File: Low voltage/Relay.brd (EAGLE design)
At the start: 100 x 80 mm, 9 parts, among them T1 2N1613

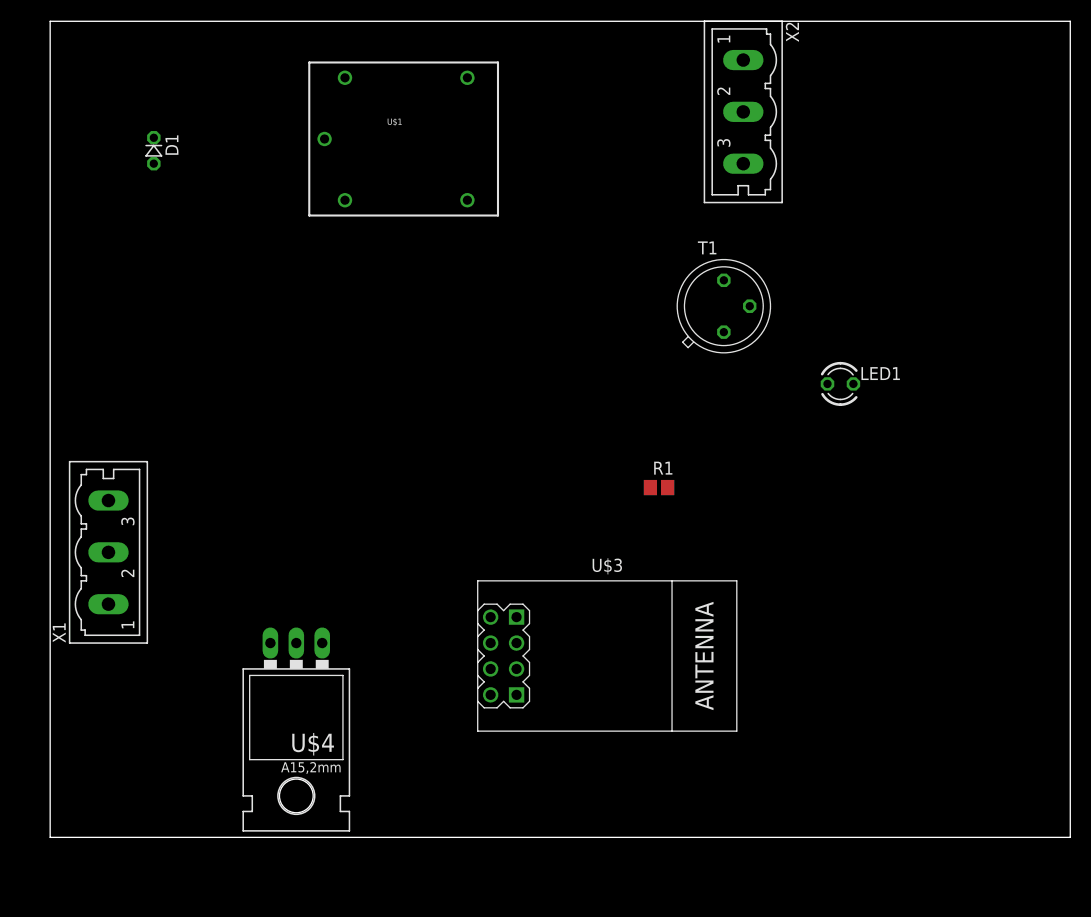
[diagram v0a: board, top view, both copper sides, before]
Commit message: board layout
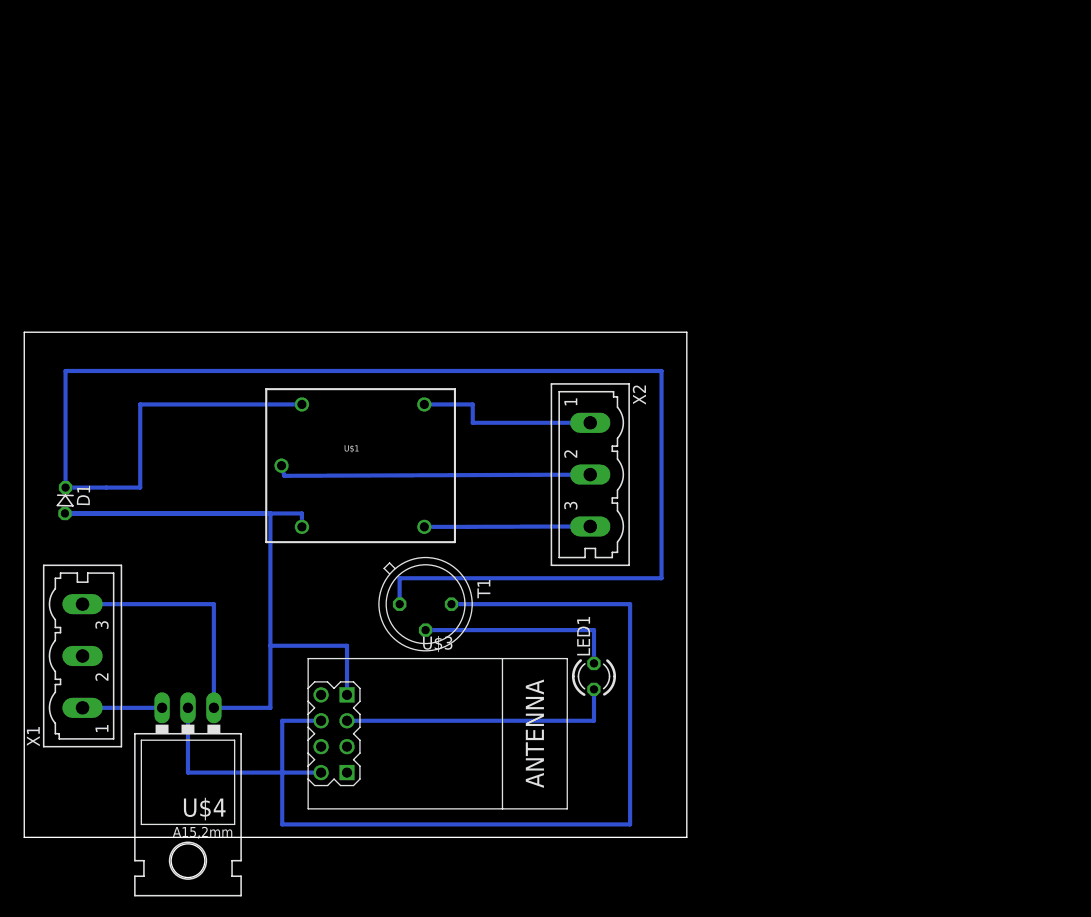
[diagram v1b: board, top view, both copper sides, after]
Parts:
- removed R1: 1k, resistor:R2012
- moved T1 41.3 mm to (36.8, 22.9), turned to 270 degrees
- moved X2 38.6 mm to (53.6, 35.6)
- moved LED1 37.5 mm to (53.3, 15.8), turned to 90 degrees
- moved D1 35.4 mm to (1.48, 33.0), turned to 268.7 degrees
- moved U$1 32.3 mm to (30.1, 36.6)
- moved U$3 18.3 mm to (38.0, 10.2)
- moved U$4 12.4 mm to (13.5, 8.89)
- moved X1 10.5 mm to (2.54, 17.8)
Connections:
- removed net N$3: LED1.A, R1.2
- net N$2: now also LED1.A; no longer R1.1
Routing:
- net N$8: track 0.00 -> 149.7 mm
- net N$1: track 0.00 -> 106.6 mm
- net GND: track 0.00 -> 104.6 mm
- net N$9: track 0.00 -> 31.0 mm
- net N$2: track 0.00 -> 27.3 mm
- net N$5: track 0.00 -> 19.8 mm
- net N$10: track 0.00 -> 18.1 mm
- net N$7: track 0.00 -> 16.3 mm
- net N$4: track 0.00 -> 7.80 mm
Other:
- board size 100 x 80 mm -> 65 x 49.5 mm
